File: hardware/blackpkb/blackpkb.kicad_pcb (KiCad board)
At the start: 2 copper layers, 96 x 96 mm, 32 parts, among them SW1 SW_Push_45deg, SW10 SW_Push_45deg, SW11 SW_Push_45deg, SW12 SW_Push_45deg, SW13 RotaryEncoder_Switch, SW2 SW_Push_45deg, SW3 SW_Push_45deg, SW4 SW_Push_45deg, SW5 SW_Push_45deg, SW6 SW_Push_45deg, SW7 SW_Push_45deg, SW8 SW_Push_45deg, SW9 SW_Push_45deg, U1 YAAJ_WeAct_BlackPill_Part_Lik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

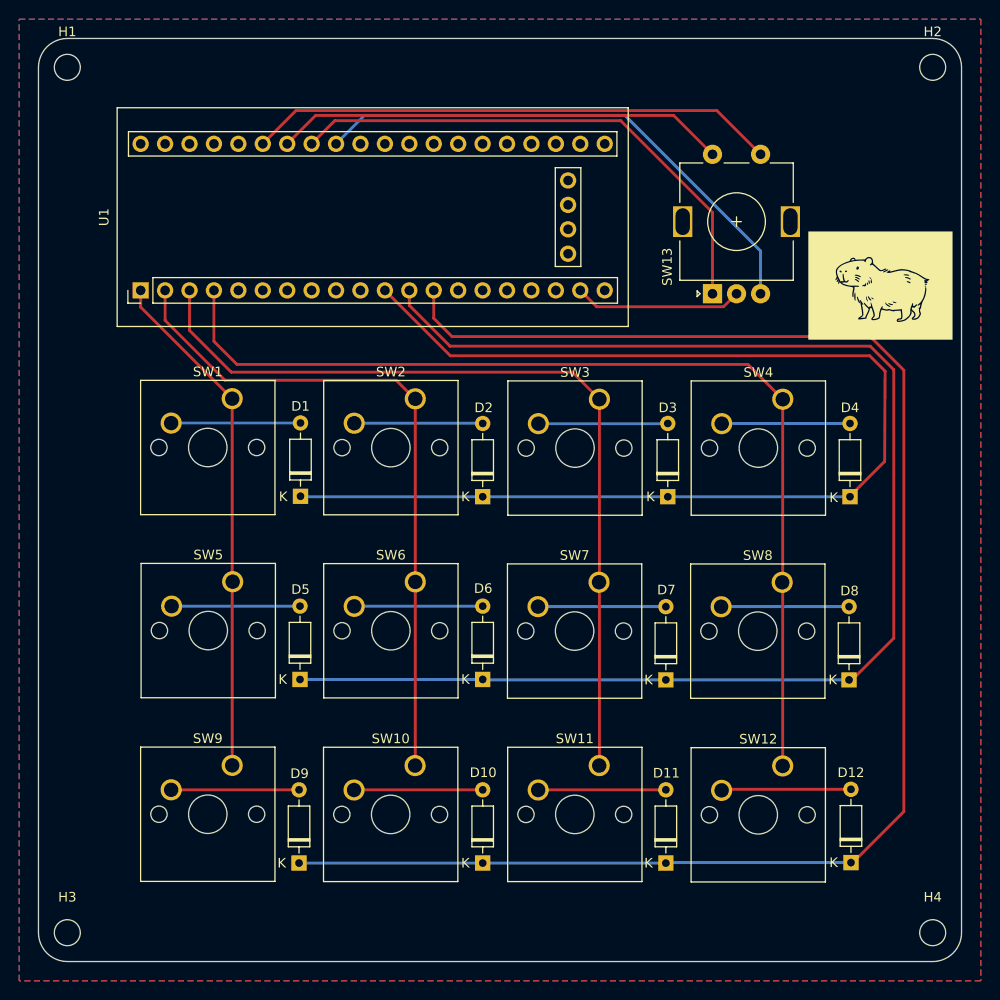
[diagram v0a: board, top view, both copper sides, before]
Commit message: hardware v0.2
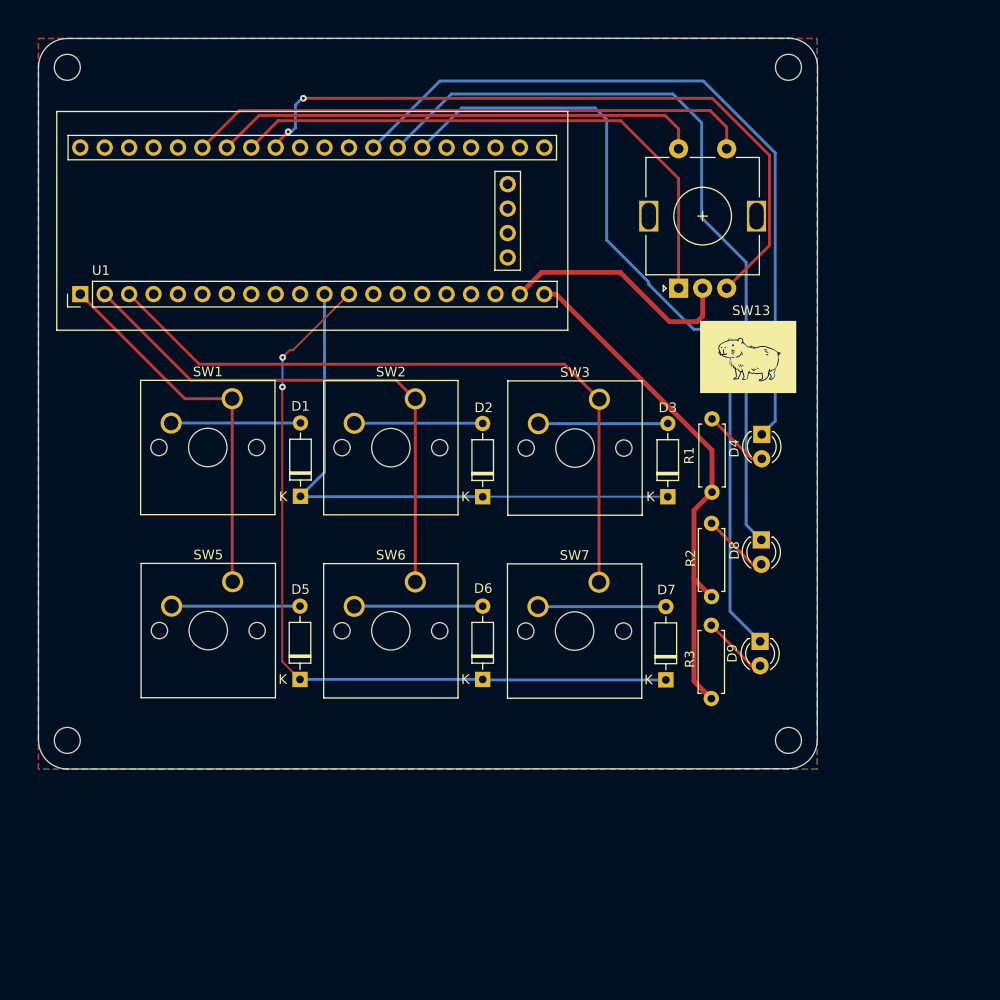
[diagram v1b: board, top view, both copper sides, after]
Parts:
- removed D10, D11, D12: 1N4148, Diode_THT:D_DO-35_SOD27_P7.62mm_Horizontal
- removed SW10, SW11, SW12, SW4, SW8, SW9: SW_Push_45deg, Button_Switch_Keyboard:SW_Cherry_MX_1.00u_PCB
- added R1: 330, Resistor_THT:R_Axial_DIN0207_L6.3mm_D2.5mm_P7.62mm_Horizontal, F.Cu at (202.1, 64.2)
- added R2: 330, Resistor_THT:R_Axial_DIN0207_L6.3mm_D2.5mm_P7.62mm_Horizontal, F.Cu at (202.0, 75.0)
- added R3: 330, Resistor_THT:R_Axial_DIN0207_L6.3mm_D2.5mm_P7.62mm_Horizontal, F.Cu at (202.0, 85.7)
- D4, D8, D9: value 1N4148 -> LED_Small; footprint Diode_THT:D_DO-35_SOD27_P7.62mm_Horizontal -> LED_THT:LED_D3.0mm
- moved D9 53.2 mm to (207.1, 79.7), turned to -90 degrees
- moved G*** 45.6 mm to (171.2, 35.6)
- moved H4 25.0 mm to (210.0, 90.0)
- moved H3 20.0 mm to (135.0, 90.0)
- moved D8 17.2 mm to (207.2, 69.2), turned to -90 degrees
- moved G*** 15.6 mm to (205.8, 50.1)
- moved H2 15.0 mm to (210.0, 20.0)
- moved D4 11.2 mm to (207.2, 58.2), turned to -90 degrees
- moved U1 6.29 mm to (136.3, 43.6)
- moved SW13 3.57 mm to (198.6, 43.0)
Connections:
- D4 pad 1: /ROW_1 -> /LED_YELLOW
- D8 pad 1: /ROW_2 -> /LED_GREEN
- D9 pad 1: /ROW_3 -> /LED_RED
- U1 pad 13: /ROW_3 -> unconnected-(U1-PB5-Pad13)
- U1 pad 20: unconnected-(U1-3V3-Pad20) -> +3.3V
- U1 pad 26: unconnected-(U1-PA0-Pad26) -> /LED_RED
- U1 pad 27: unconnected-(U1-PA1-Pad27) -> /LED_GREEN
- U1 pad 28: unconnected-(U1-PA2-Pad28) -> /LED_YELLOW
- U1 pad 4: /COL_4 -> unconnected-(U1-PB15-Pad4)
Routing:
- net /ROW_3: track 165.1 -> 0.00 mm
- net /COL_4: track 105.1 -> 0.00 mm
- net /LED_RED: track 0.00 -> 84.0 mm
- net /LED_GREEN: track 0.00 -> 81.1 mm
- net /LED_YELLOW: track 0.00 -> 77.6 mm
- net /ROW_1: track 127.2 -> 60.3 mm
- net /ROW_2: track 146.2 -> 82.0 mm, vias 0 -> 2
- net +3.3V: track 0.00 -> 54.2 mm
- net /ENCODER_B: track 55.7 -> 73.2 mm, vias 0 -> 2
- net /COL_3: track 87.9 -> 72.5 mm
- net /COL_2: track 70.7 -> 55.9 mm
- net /COL_1: track 53.3 -> 39.4 mm
- net Net-(D12-A): track 13.5 -> 0.00 mm
- net Net-(D10-A): track 13.4 -> 0.00 mm
- net Net-(D11-A): track 13.3 -> 0.00 mm
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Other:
- board size 96 x 96 mm -> 81 x 76 mm
- board text added: "bluepkb 07/24 - v0.2 alcato"
- board text removed: "author - alcato"
- board text removed: "bluepkb"
- board text removed: "v0.1"
